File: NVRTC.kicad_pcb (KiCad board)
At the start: 2 copper layers, 26.4 x 38.1 mm, 4 parts

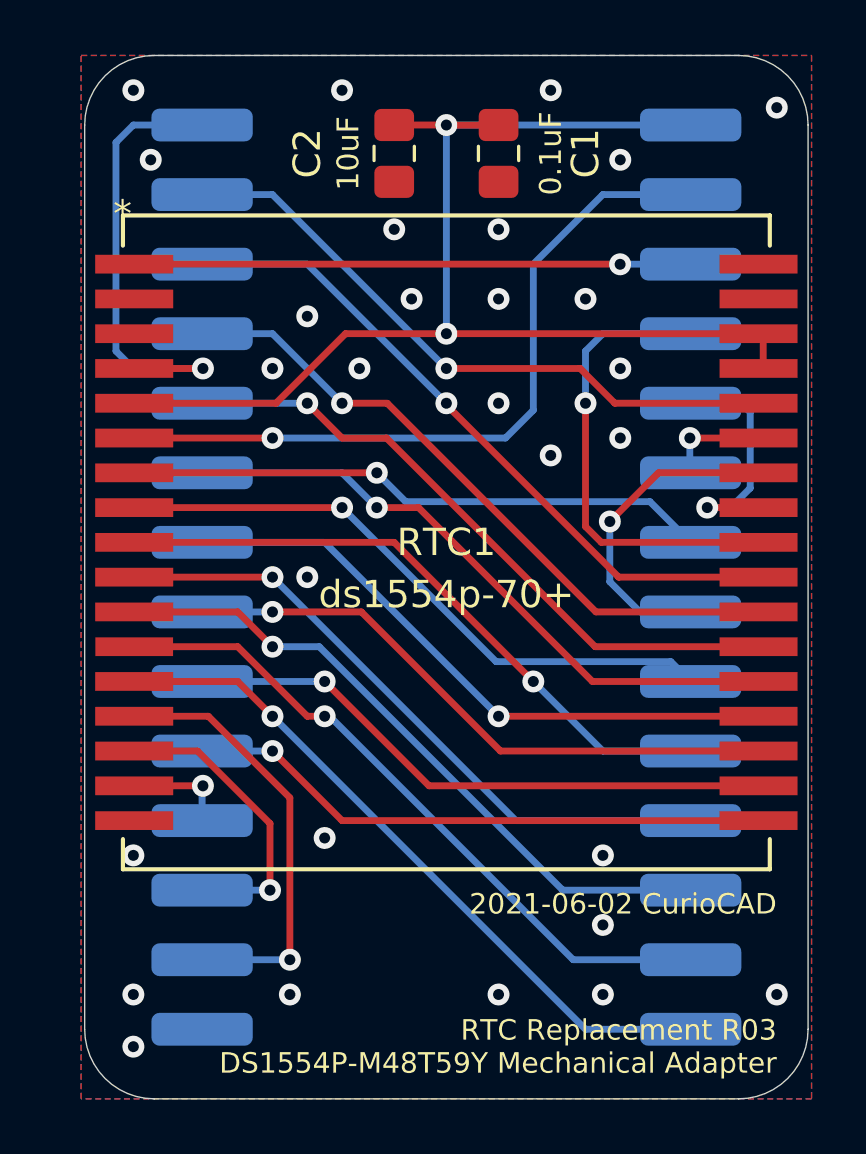
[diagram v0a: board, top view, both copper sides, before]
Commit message: Rev 4
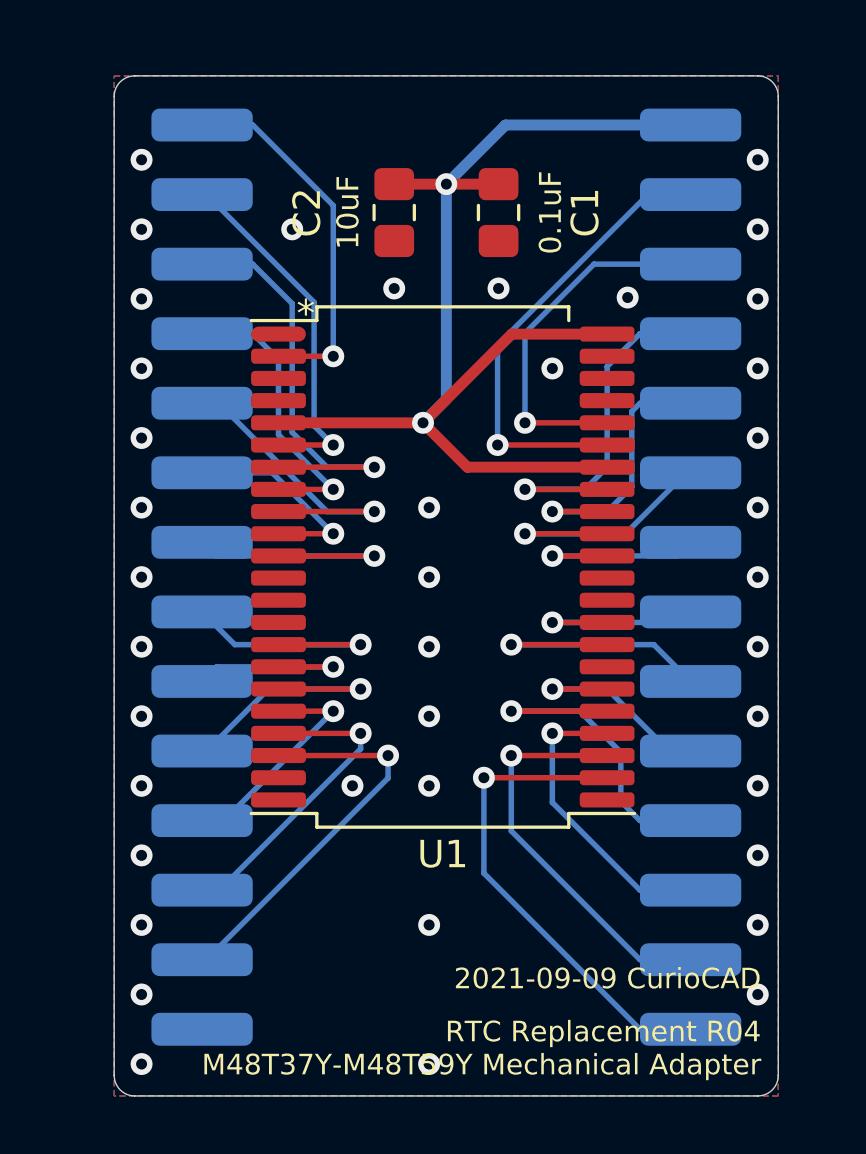
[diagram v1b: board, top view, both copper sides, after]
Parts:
- removed RTC1: ds1554p-70+, lib_fp:ds1554p-70+rev2
- added U1: M48T37Y, lib_fp:STM-SOH-44, F.Cu at (151.0, 92.3)
- moved C1 2.16 mm to (153.0, 79.4)
- moved C2 2.16 mm to (149.2, 79.4)
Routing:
- net /A4: track 23.6 -> 7.71 mm
- net /D7: track 23.6 -> 7.99 mm
- net /A1: track 22.1 -> 7.38 mm
- net /OutputEnable: track 21.5 -> 7.26 mm
- net /A6: track 24.7 -> 10.8 mm
- net /D5: track 24.7 -> 10.9 mm
- net /A2: track 22.6 -> 9.28 mm
- net /A3: track 23.1 -> 10.00 mm
- net /A5: track 24.2 -> 11.4 mm
- net /ChipEnable: track 23.1 -> 10.6 mm
- net /A0: track 22.3 -> 10.4 mm
- net /D6: track 24.2 -> 12.8 mm
- net /D4: track 25.2 -> 14.8 mm
- net /A12: track 23.6 -> 13.2 mm
- net /WriteEnable: track 27.3 -> 17.0 mm
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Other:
- board size 26.4 x 38.1 mm -> 24.2 x 37.2 mm
- net class 5V added: clearance 0.2, trace_width 0.4, via_dia 0.8, via_drill 0.4
- net class Default: clearance 0.1524 -> 0.2; trace_width 0.225 -> 0.2
- rule pad_to_mask_clearance: 0.0508 -> 0
- rule trace_clearance: 0.1524 -> 0.2
- board text added: "2021-09-09 CurioCAD"
- board text added: "RTC Replacement R04 M48T37Y-M48T59Y Mechanical Adapter"
- board text removed: "2021-06-02 CurioCAD"
- board text removed: "RTC Replacement R03 DS1554P-M48T59Y Mechanical Adapter"
